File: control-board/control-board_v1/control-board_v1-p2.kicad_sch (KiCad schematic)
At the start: 20 parts, among them Q10 NMOS, Q9 NMOS, U3 ADS1118, U4 Opamp_Dual, U6 Opamp_Dual

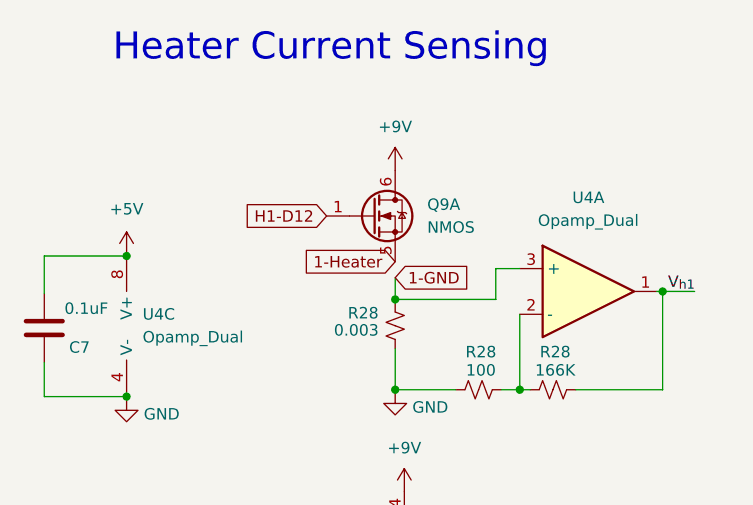
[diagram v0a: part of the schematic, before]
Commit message: additional notes
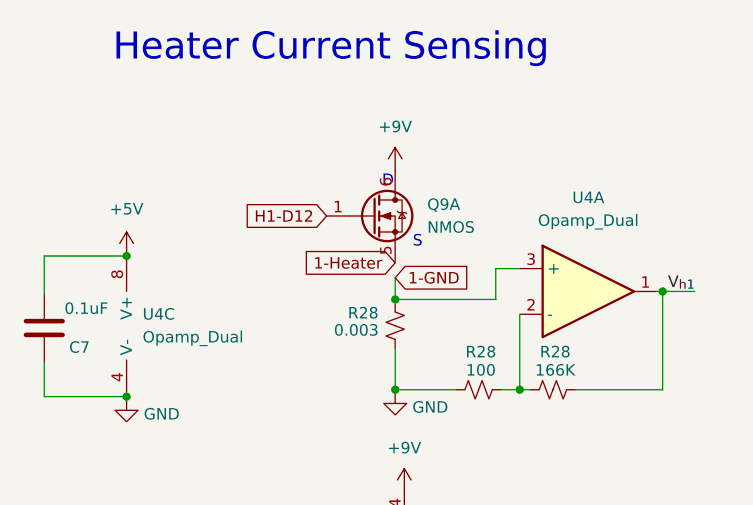
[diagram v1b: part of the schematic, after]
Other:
- note added: "D"
- note added: "S"
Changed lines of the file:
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@@
+    (stroke (width 0) (type default))
+  )
+  (wire (pts (xy 86.868 48.768) (xy 86.868 48.641))
     (stroke (width 0) (type default))
   )
@@
   (text "Heater Current Sensing" (at 55.499 26.67 0)
     (effects (font (size 3 3)) (justify left bottom))
+  )
+  (text "S" (at 89.916 47.244 0)
+    (effects (font (size 1.27 1.27)) (justify right bottom))
+  )
+  (text "D" (at 86.741 40.513 0)
+    (effects (font (size 1.27 1.27)) (justify right bottom))
   )
   (text "G = 1+ R22/R21\nG = 1 + 166k/100\nG = 1661\n\n" (at 123.952 116.205 0)
@@
     )
   )
-  (global_label "1-Heater" (shape input) (at 86.868 48.641 180) (fields_autoplaced)
+  (global_label "1-Heater" (shape input) (at 86.868 48.768 180) (fields_autoplaced)
     (effects (font (size 1.27 1.27)) (justify right))
-    (property "Intersheetrefs" "${INTERSHEET_REFS}" (at 74.9323 48.641 0)
+    (property "Intersheetrefs" "${INTERSHEET_REFS}" (at 74.9323 48.768 0)
       (effects (font (size 1.27 1.27)) (justify right) hide)
     )
